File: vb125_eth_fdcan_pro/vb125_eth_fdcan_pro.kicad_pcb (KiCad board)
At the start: 4 copper layers, 105 x 82 mm, 319 parts, among them J1 MEM2061-01-188-00-A, J2 TAGconnect NL, J3 Conn_02x20_Pin, J4 ARJM11D7-114-AB, J5 USB_C_Receptacle_USB2.0, J6 D09P33E4GL00LF, J7 D09P33E4GL00LF, K1 EE2-4.5TNUH, K2 EE2-4.5TNUH, M1 DM-OLED042-647, M2 B0505MT-1WR4, M3 B0505MT-1WR4, Q1 BSS138, Q2 BSS138, Q3 BSS138, Q4 BSS138, Q5 MMBTA42, Q6 Si3440DV, Q7 2N7002, SW1 KSS331GLFS, T1 PA1134NL, T2 750315125, U1 STM32H725IGKx, U10 TLP2270, U11 LTC4267, U12 PS2911-1-F3-AX, U13 ZR431, U15 LT8304IS8E#PBF, U2 LAN8740A, U3 NCP563SQ18T1G, U4 USB3315, U5 AOZ1376DI-02, U6 RT5760A/B, U7 ADM3050EBRIZ, U8 TLP2270, U9 ADM3050EBRIZ, X1 ECX-.327-CDX-1293, X2 50MHz, X3 24MHz

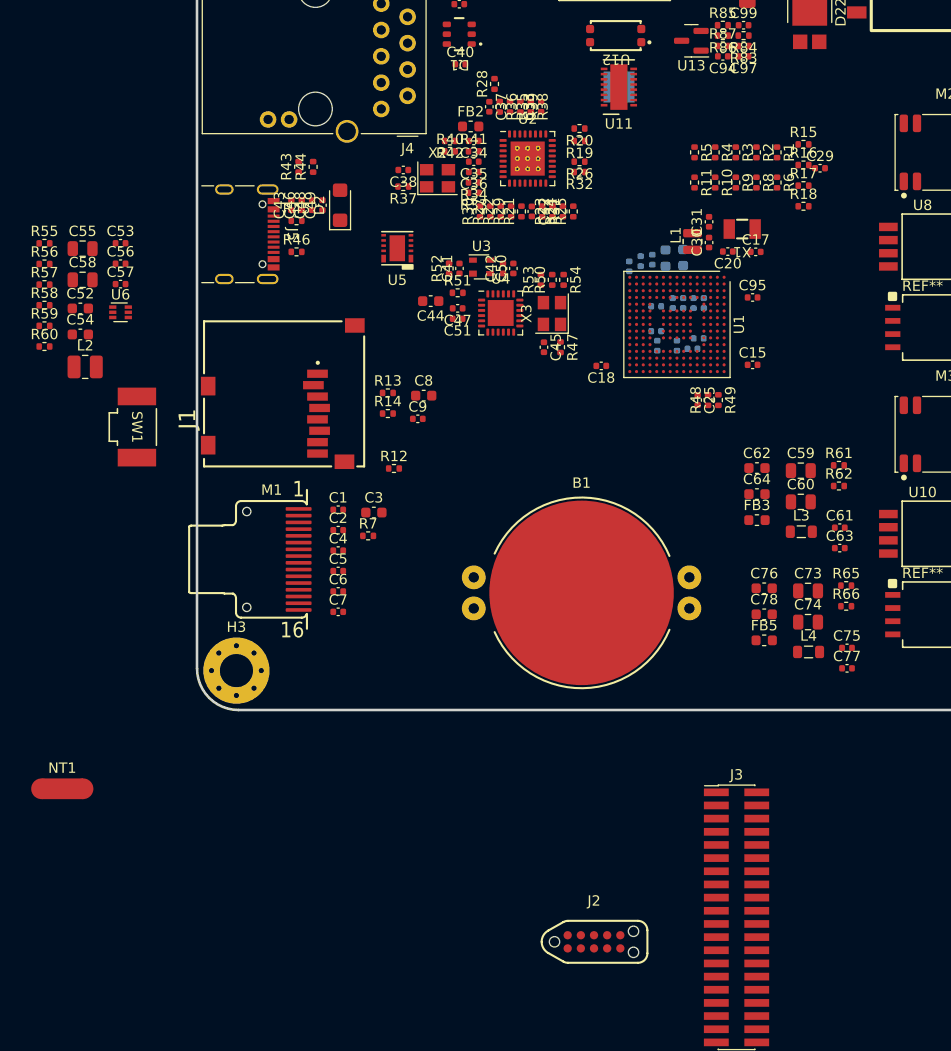
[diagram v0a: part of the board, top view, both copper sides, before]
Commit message: Continue with floorplan
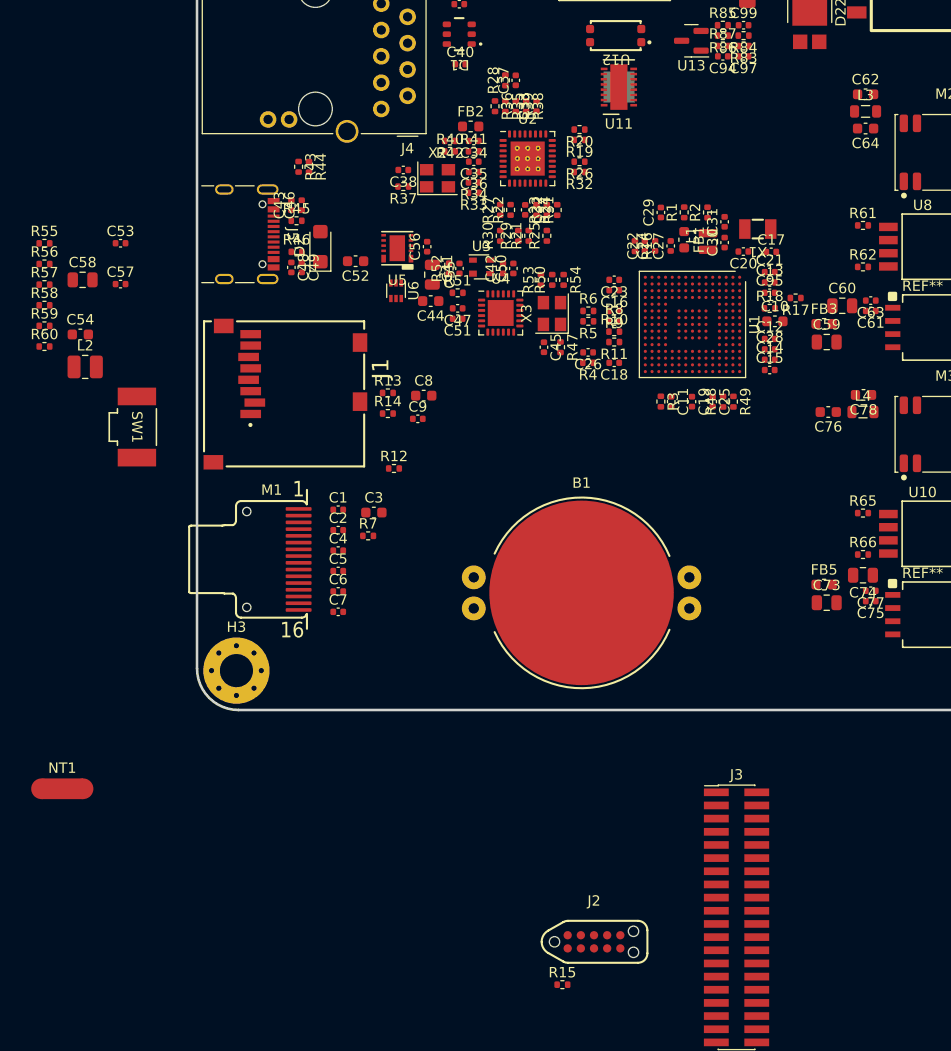
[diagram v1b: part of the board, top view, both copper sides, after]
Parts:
- C10, C11, C12, C13, C14, C16, C19, C21, C22, C23, C24, C26, C27, C28, FB1: moved to F.Cu
- moved R15 84.3 mm to (132.2, 165.5)
- moved L3 41.0 mm to (161.5, 81.2)
- moved C62 37.6 mm to (161.5, 79.6)
- moved C64 36.8 mm to (161.5, 82.9), turned to 180 degrees
- moved C55 33.8 mm to (119.7, 97.0), turned to -90 degrees
- moved C56 29.6 mm to (119.2, 94.3), turned to 90 degrees
- moved C52 26.9 mm to (112.3, 95.7), turned to 180 degrees
- moved U6 26.7 mm to (116.2, 98.5), turned to -90 degrees
- moved R3 25.1 mm to (141.8, 109.2)
- moved C63 24.1 mm to (162.0, 99.5), turned to 180 degrees
- moved L4 23.7 mm to (161.2, 110.2)
- moved R4 23.7 mm to (134.7, 105.5), turned to 180 degrees
- moved R61 23.3 mm to (161.2, 92.2)
- moved C78 23.2 mm to (161.3, 108.6), turned to 180 degrees
- moved R6 22.0 mm to (134.8, 100.5), turned to 0 degrees
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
